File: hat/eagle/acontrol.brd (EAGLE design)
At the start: 65.3 x 30.7 mm, 8 parts, among them J1 RASPBERRYPI-40-PIN-GPIO_PTH_N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, J4 4P-2.0-90D, J5 GREEN-2P-3.5, J7 455-1750-1-ND, U1 TXB0104

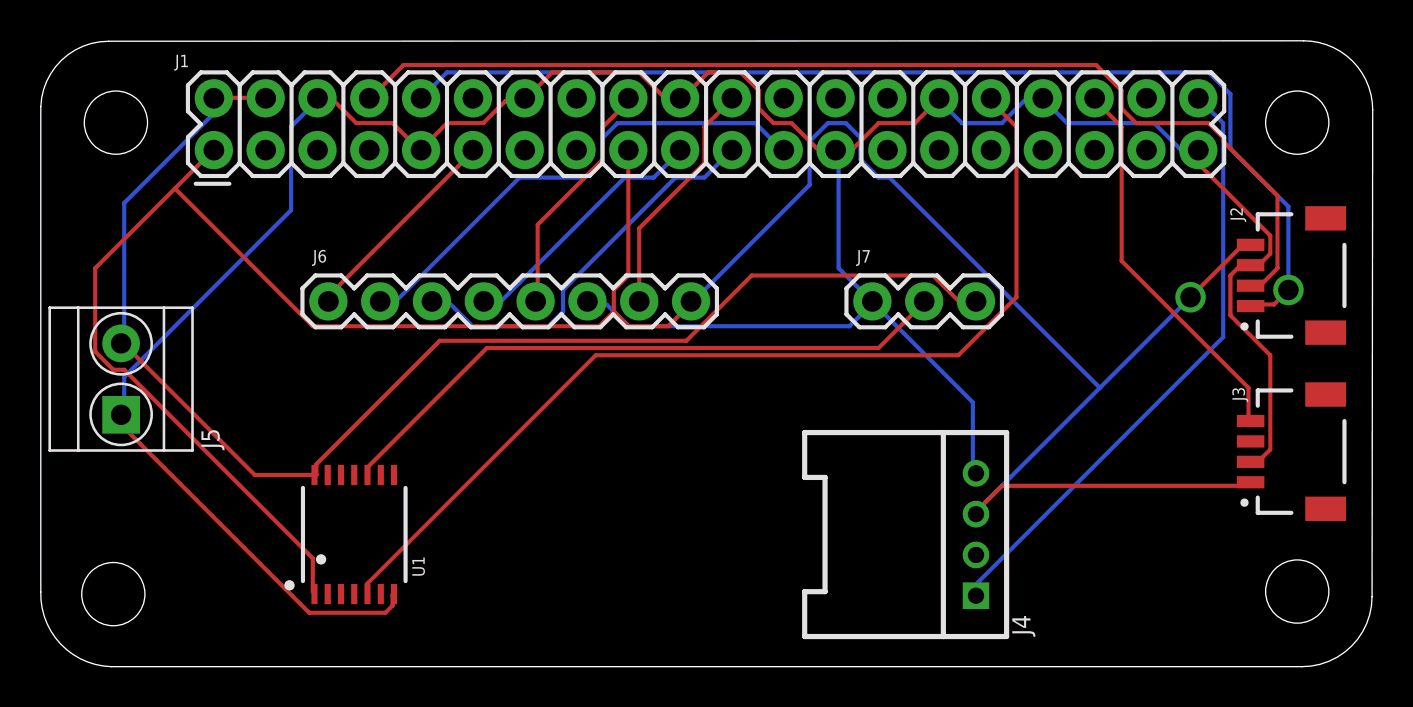
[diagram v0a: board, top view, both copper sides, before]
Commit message: hardware - Raspberry PI Zero W uHat
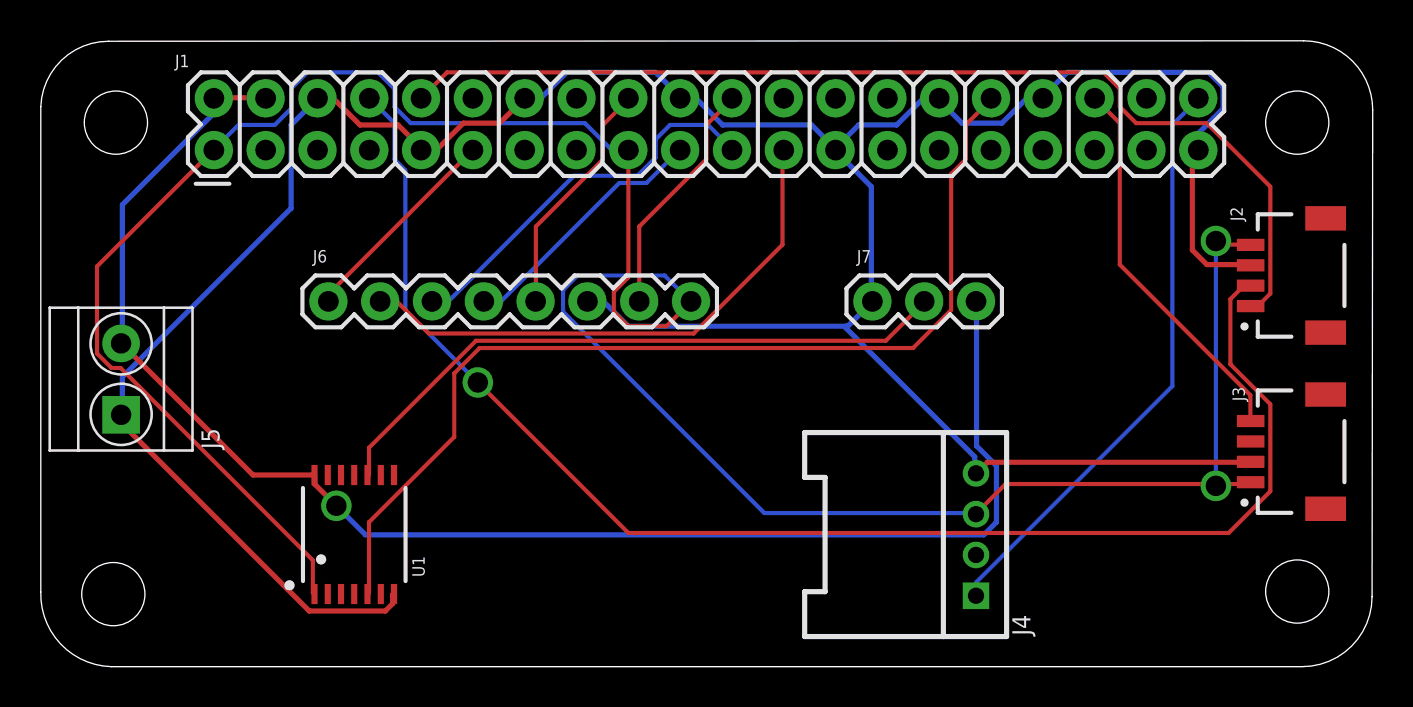
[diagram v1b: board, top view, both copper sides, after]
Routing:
- net GT_RX: track 53.7 -> 70.4 mm, vias 0 -> 1
- net 5V: track 65.9 -> 75.0 mm, vias 0 -> 1
- net GND: track 143.5 -> 148.0 mm
- net 3.3V: track 130.5 -> 126.8 mm, vias 1 -> 2
- net MFRC522_SCK: track 24.6 -> 26.9 mm
- net GT_TX: track 53.6 -> 51.5 mm, vias 1 -> 0
- net BUZZER_IN: track 29.9 -> 28.9 mm
- net NEOPIXEL_IN: track 48.4 -> 49.4 mm
- net NEOPIXEL_OUT: track 31.1 -> 31.6 mm
